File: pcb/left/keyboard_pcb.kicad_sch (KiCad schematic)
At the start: 52 parts, among them J1 TRRS, K0 KEYSW, K1 KEYSW, K10 KEYSW, K11 KEYSW, K12 KEYSW, K13 KEYSW, K14 KEYSW, K15 KEYSW, K2 KEYSW, K20 KEYSW, K21 KEYSW, K22 KEYSW, K23 KEYSW, K24 KEYSW, K25 KEYSW, K3 KEYSW, K30 KEYSW, K31 KEYSW, K32 KEYSW, K4 KEYSW, K5 KEYSW, U1 MCP23009-E/SO, U2 Pico, U3 PCF8574TS

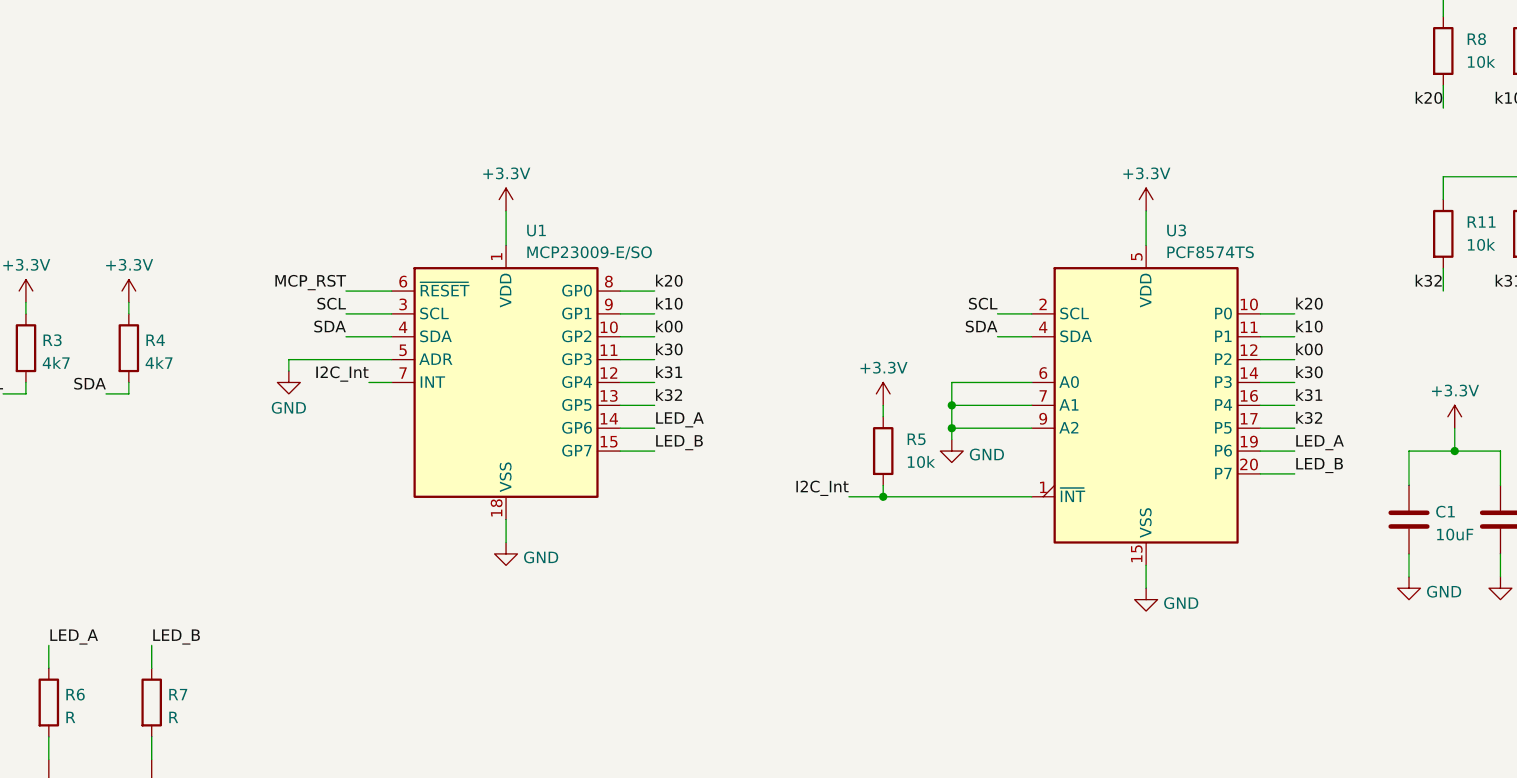
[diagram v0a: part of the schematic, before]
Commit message: Left side routing wip
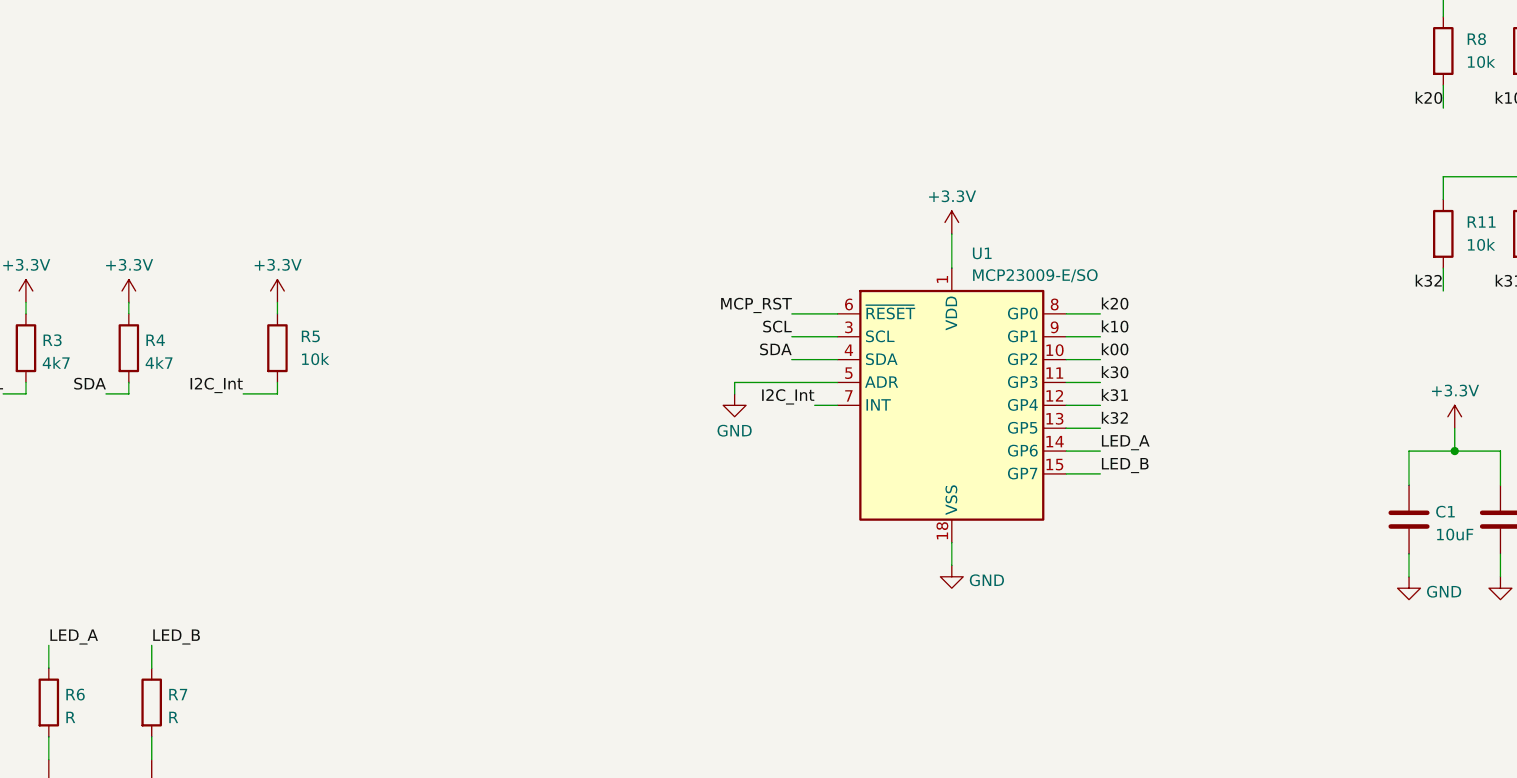
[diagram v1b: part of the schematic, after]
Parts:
- removed U3: PCF8574TS, Package_SO:SSOP-20_4.4x6.5mm_P0.65mm, symbol Interface_Expansion:PCF8574TS
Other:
- moved on the sheet: R5, U1
